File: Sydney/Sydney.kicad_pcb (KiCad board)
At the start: 2 copper layers, 54 x 87.6 mm, 5 parts, among them J1 Conn_01x02_Pin, U1 NT3H2111W0FHKH

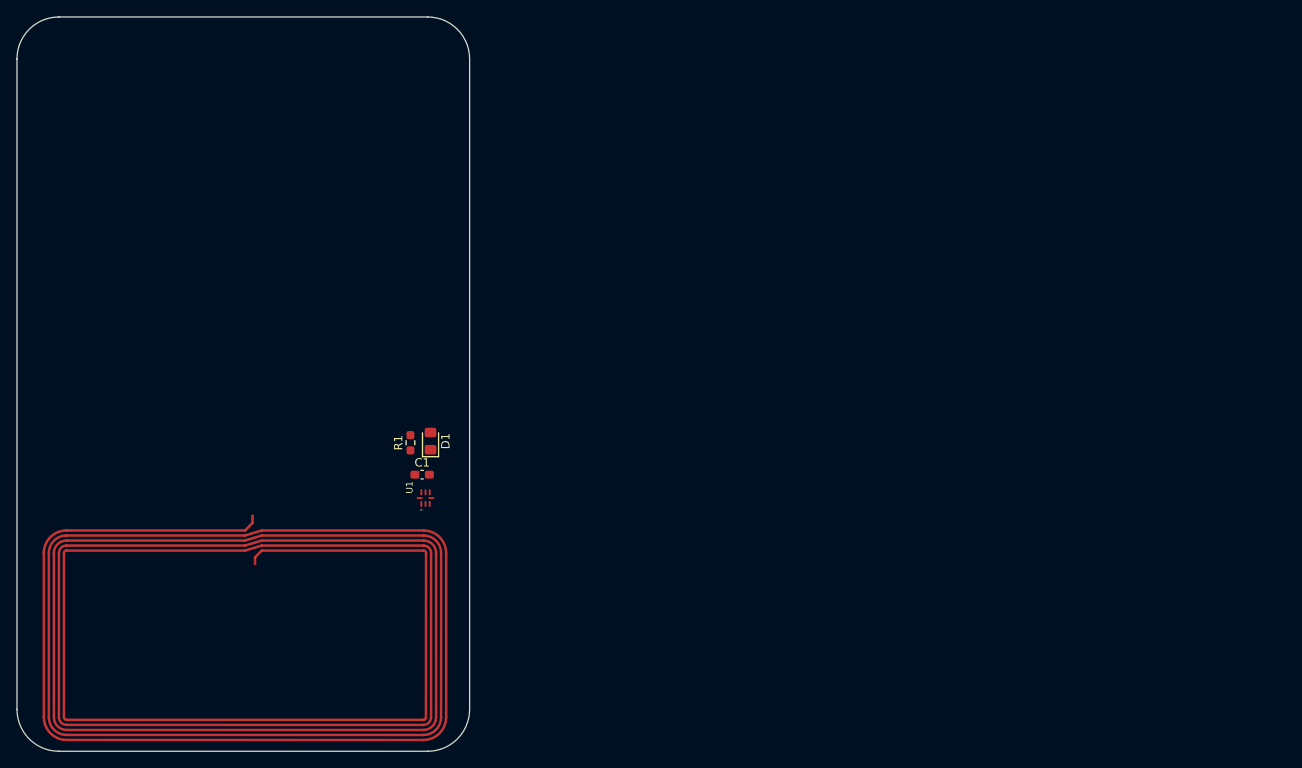
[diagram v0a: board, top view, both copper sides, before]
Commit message: lots of stuff
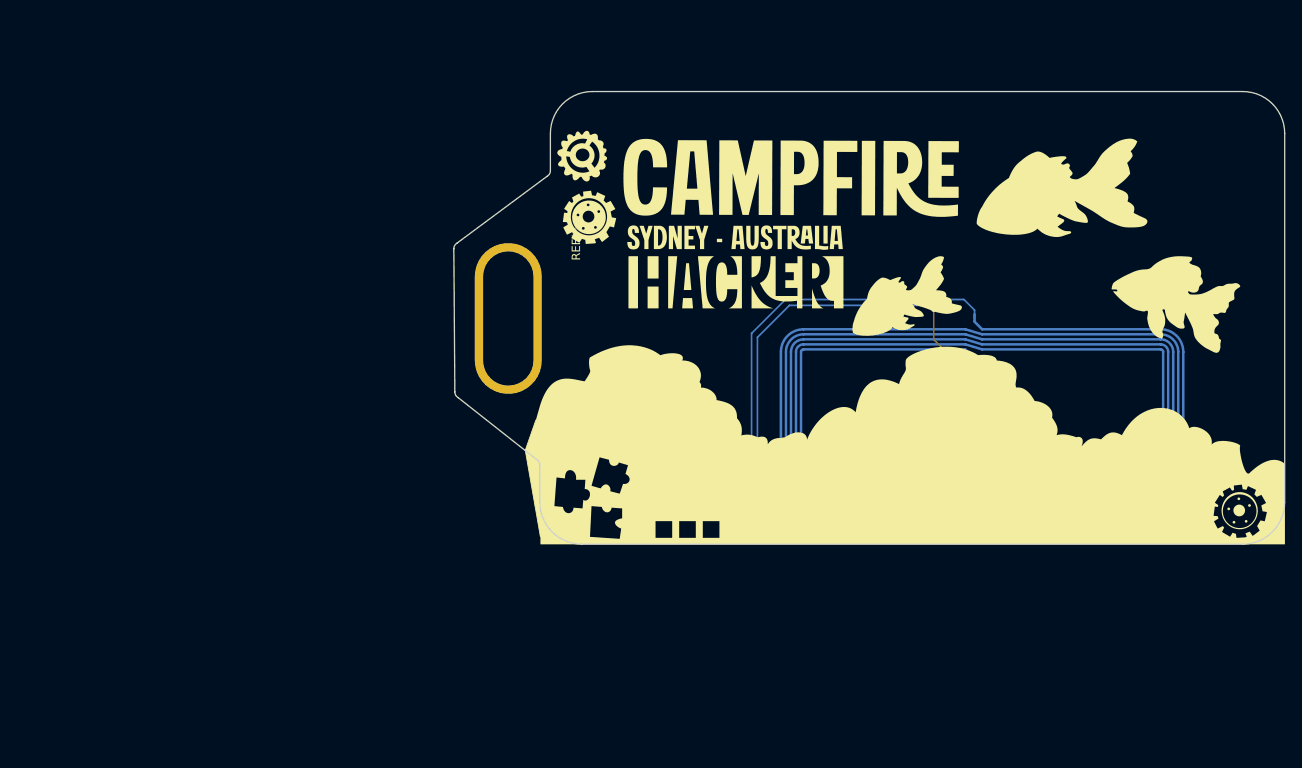
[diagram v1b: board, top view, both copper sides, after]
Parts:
- added REF**: Lanyard hole, Taranium-libs:Lanyard hole, F.Cu at (169.4, 65.2)
- C1, D1, J1, R1, U1: moved to B.Cu
- moved J1 91.2 mm to (217.3, 87.9), turned to 180 degrees
- moved U1 38.9 mm to (189.8, 95.5), turned to 180 degrees
- moved C1 36.6 mm to (187.0, 95.1), turned to -90 degrees
- moved R1 34.4 mm to (183.2, 93.7), turned to 180 degrees
- moved D1 32.4 mm to (183.0, 96.1), turned to 180 degrees
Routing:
- net Net-(J1-Pin_2): track 0.00 -> 51.3 mm, vias 0 -> 2
- net Net-(J1-Pin_1): track 0.00 -> 48.4 mm
- net Net-(D1-K): track 0.00 -> 9.92 mm
- net Net-(U1-VCC): track 0.00 -> 6.03 mm
- net Net-(D1-A): track 0.00 -> 2.53 mm
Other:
- board size 54 x 87.6 mm -> 99.1 x 54 mm
